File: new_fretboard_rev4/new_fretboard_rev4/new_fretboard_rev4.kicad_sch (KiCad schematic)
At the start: 48 parts, among them J1 Conn_01x06, J2 Conn_01x06, U1 LX3302AQPW_TSSOP-14, U2 LX3302AQPW_TSSOP-14

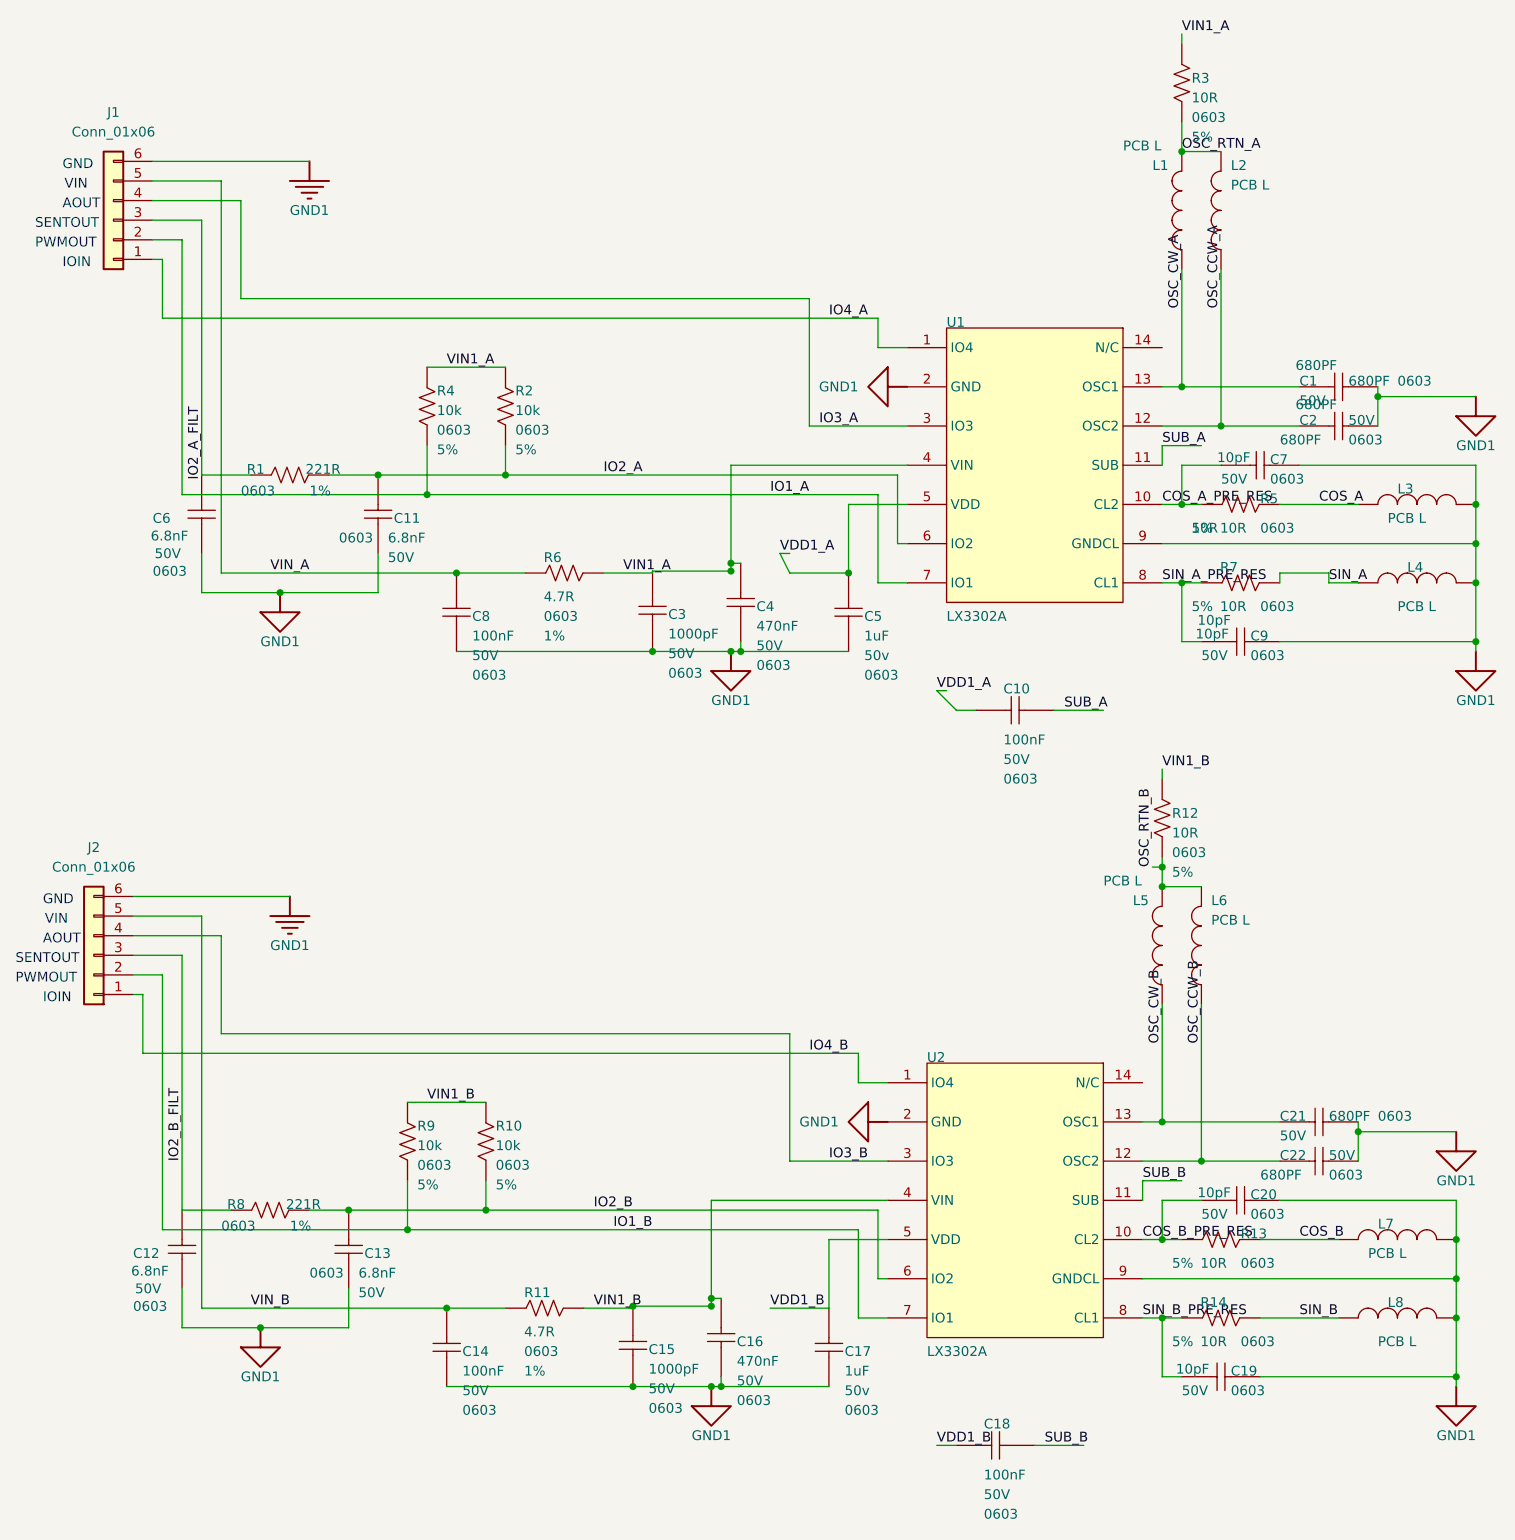
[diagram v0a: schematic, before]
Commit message: two channels done
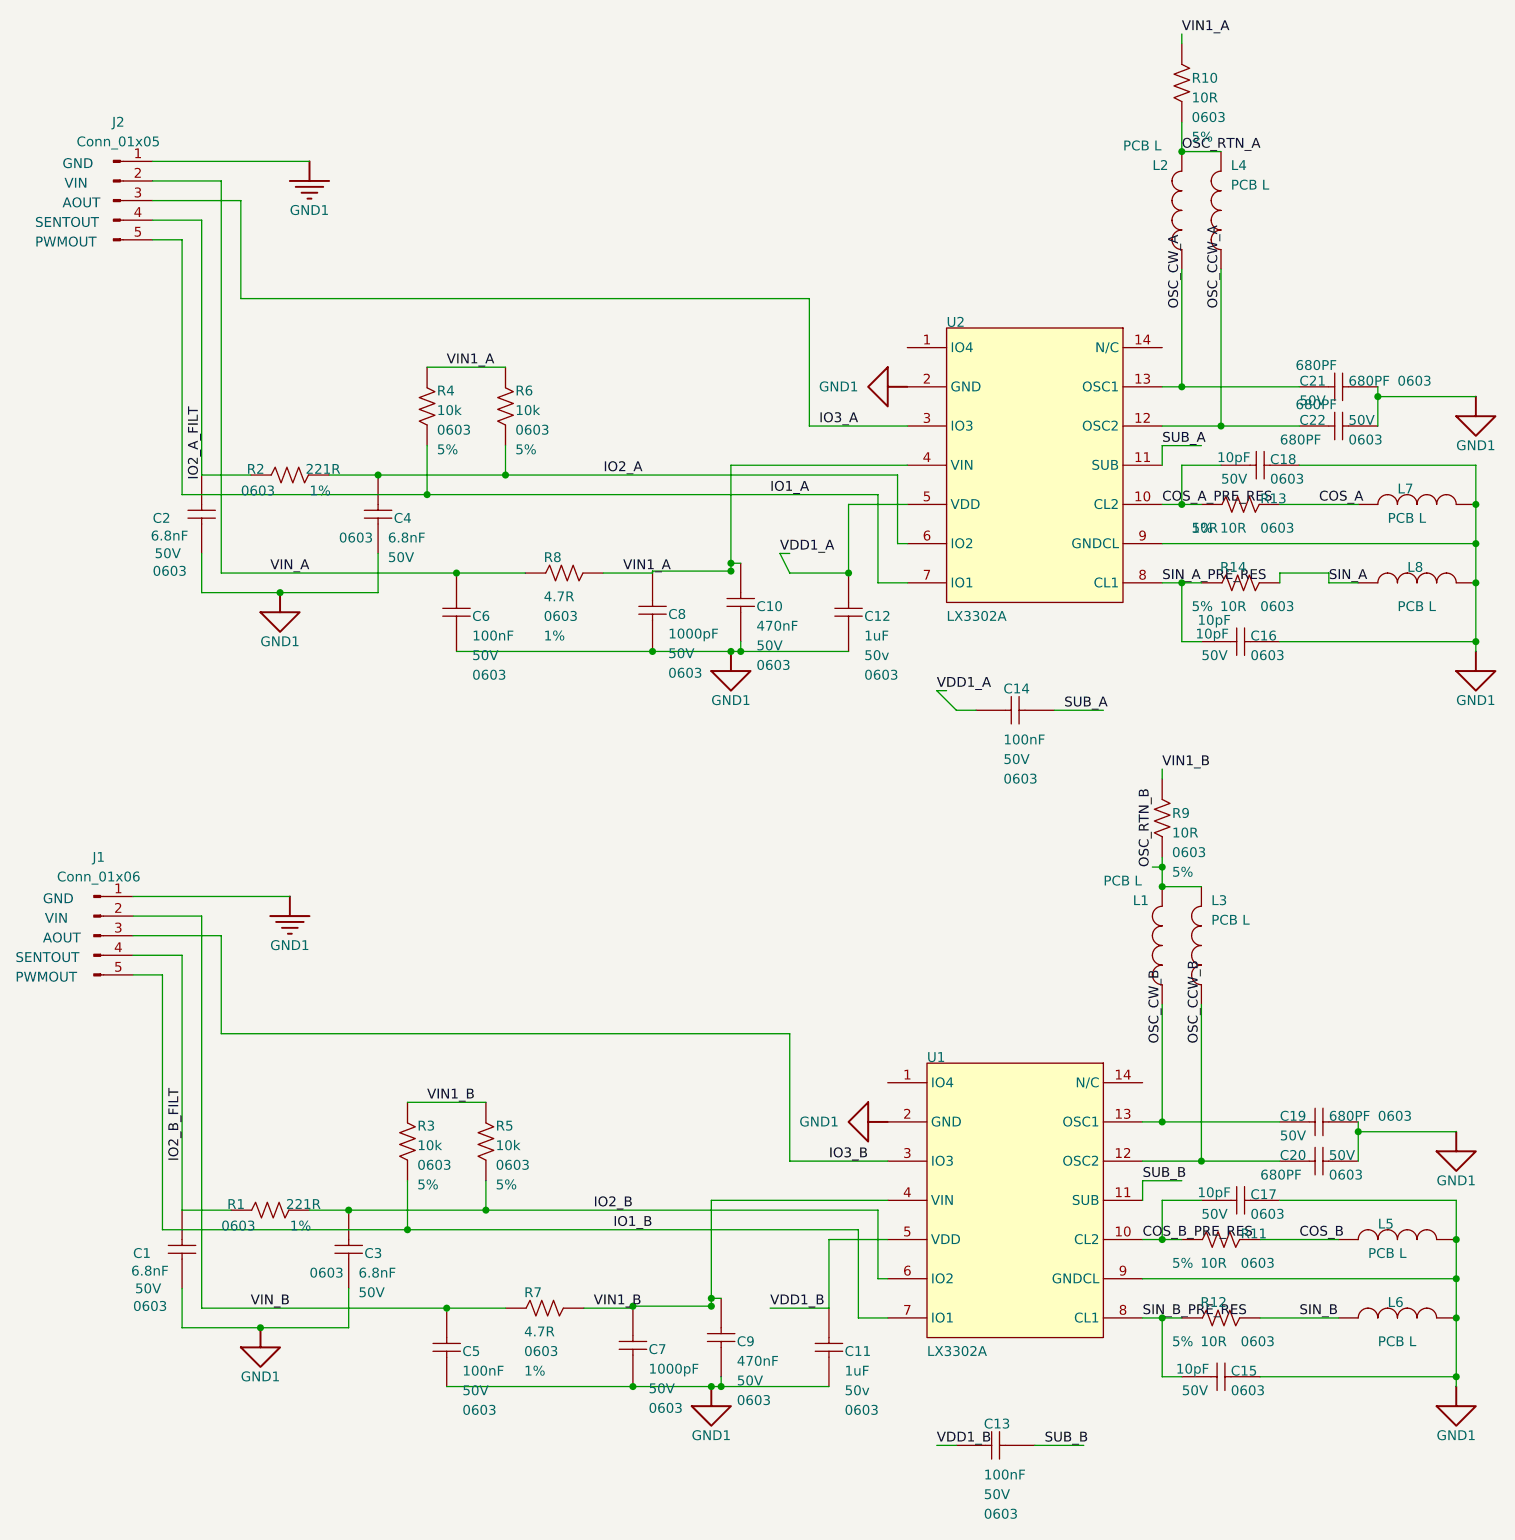
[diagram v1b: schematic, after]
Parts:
- J1: renamed from J2; footprint Connector_PinHeader_2.54mm:PinHeader_1x06_P2.54mm_Vertical -> Connector_PinHeader_2.54mm:PinHeader_1x05_P2.54mm_Vertical; symbol PCM_4ms_Connector:Conn_01x06 -> Connector:Conn_01x05_Pin; Specifications HEADER 1x6 MALE PINS 0.100” 180deg -> HEADER 1x5 MALE PINS 0.100” 180deg
- J2: renamed from J1; value Conn_01x06 -> Conn_01x05; footprint Connector_PinHeader_2.54mm:PinHeader_1x06_P2.54mm_Vertical -> Connector_PinHeader_2.54mm:PinHeader_1x05_P2.54mm_Vertical; symbol PCM_4ms_Connector:Conn_01x06 -> Connector:Conn_01x05_Pin; Specifications HEADER 1x6 MALE PINS 0.100” 180deg -> HEADER 1x5 MALE PINS 0.100” 180deg
- renumbered C12 to C1, C4 to C10, C17 to C11, C5 to C12, C18 to C13, C10 to C14, C19 to C15, C9 to C16, C20 to C17, C7 to C18, C21 to C19, C6 to C2, C22 to C20, C1 to C21, C2 to C22, C13 to C3, C11 to C4, C14 to C5, C8 to C6, C15 to C7, C3 to C8, C16 to C9, L5 to L1, L1 to L2, L6 to L3, L2 to L4, L7 to L5, L8 to L6, L3 to L7, L4 to L8, R8 to R1, R3 to R10, R13 to R11, R14 to R12, R5 to R13, R7 to R14, R1 to R2, R9 to R3, R10 to R5, R2 to R6, R11 to R7, R6 to R8, R12 to R9, U2 to U1, U1 to U2
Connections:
- net GND1: now also J1.1 (Pin_1), J2.1 (Pin_1); no longer J1.6 (Pin_6), J2.6 (Pin_6)
- net IO1_A: now also J2.5 (Pin_5); no longer J2.2 (Pin_2)
- net IO1_B: now also J1.5 (Pin_5); no longer J1.2 (Pin_2)
- net IO2_A_FILT: now also J2.4 (Pin_4); no longer J2.3 (Pin_3)
- net IO2_B_FILT: now also J1.4 (Pin_4); no longer J1.3 (Pin_3)
- net IO3_A: now also J2.3 (Pin_3); no longer J2.4 (Pin_4)
- net IO3_B: now also J1.3 (Pin_3); no longer J1.4 (Pin_4)
- net VIN_A: now also J2.2 (Pin_2); no longer J2.5 (Pin_5)
- net VIN_B: now also J1.2 (Pin_2); no longer J1.5 (Pin_5)
- net IO4_A: no longer names the net of U2.1 (IO4)
- net IO4_A: no longer J2.1 (Pin_1)
- net IO4_B: no longer names the net of U1.1 (IO4)
- net IO4_B: no longer J1.1 (Pin_1)
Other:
- note removed: "IOIN"
